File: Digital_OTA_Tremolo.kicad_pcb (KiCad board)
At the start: 2 copper layers, 1 part

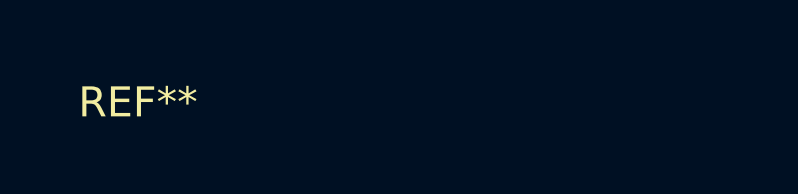
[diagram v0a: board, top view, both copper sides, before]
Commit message: updates
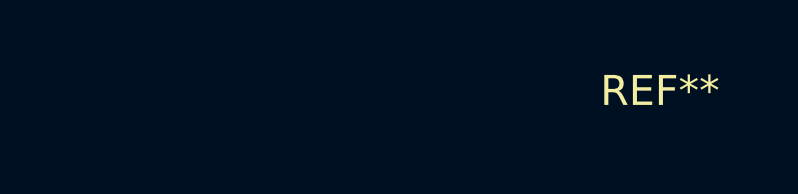
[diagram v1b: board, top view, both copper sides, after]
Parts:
- moved REF** 17.4 mm to (159.1, 99.7)
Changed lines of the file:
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@@
     (uvia_drill 0.1)
   )
-  (module Hammond1590:1590BB locked (layer F.Cu)
-    (at 141.732 100.076)
+  (module Hammond1590:1590BB (layer F.Cu)
+    (at 159.131 99.695)
     (descr "Inside Lid Width and Inside Box Height - https://www.hammfg.com/files/parts/pdf/1590BB.pdf")
     (fp_text reference REF** (at 1.27 -56.134) (layer F.SilkS)
@@
       (effects (font (size 1 1) (thickness 0.15)))
     )
-    (fp_line (start 42.037 51.689) (end 42.037 -51.308) (layer Dwgs.User) (width 0.12))
-    (fp_line (start -42.037 51.689) (end -42.037 -51.308) (layer Dwgs.User) (width 0.12))
+    (fp_line (start 42.037 51.689) (end 42.037 -48.387) (layer Dwgs.User) (width 0.12))
+    (fp_line (start -42.037 51.689) (end -42.037 -48.387) (layer Dwgs.User) (width 0.12))
     (fp_line (start -42.037 51.689) (end 42.037 51.689) (layer Dwgs.User) (width 0.12))
-    (fp_line (start -42.037 -51.308) (end 42.037 -51.308) (layer Dwgs.User) (width 0.12))
+    (fp_line (start -42.037 -48.387) (end 42.037 -48.387) (layer Dwgs.User) (width 0.12))
   )
 )
